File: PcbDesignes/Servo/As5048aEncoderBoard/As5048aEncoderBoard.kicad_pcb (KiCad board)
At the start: 2 copper layers, 8.1 x 11 mm, 8 parts, among them U1 AS5048A-HTSP-500

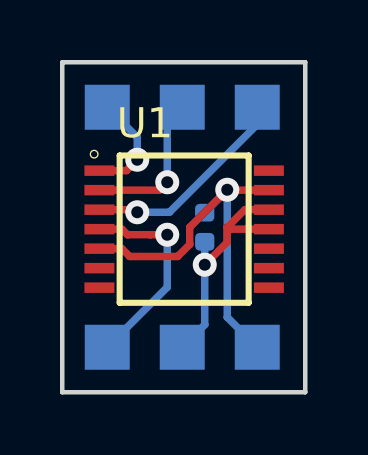
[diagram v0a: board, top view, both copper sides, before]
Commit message: updated schematics and PCB
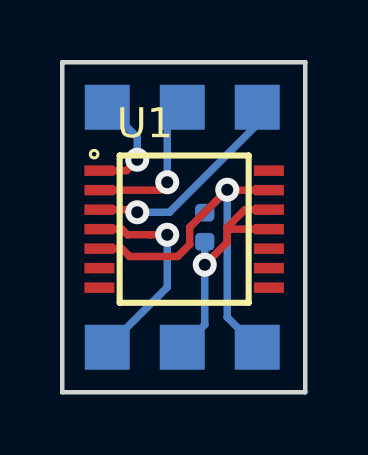
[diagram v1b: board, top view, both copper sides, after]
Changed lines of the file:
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@@
-(kicad_pcb (version 20171130) (host pcbnew 5.0.2+dfsg1-1)
+(kicad_pcb (version 20171130) (host pcbnew 5.1.5+dfsg1-2build2)
   (general
     (thickness 1.6)
@@
     (zone_45_only no)
     (trace_min 0.2)
-    (segment_width 0.2)
-    (edge_width 0.15)
     (via_size 0.8)
     (via_drill 0.4)
@@
     (uvia_min_size 0.2)
     (uvia_min_drill 0.1)
+    (edge_width 0.15)
+    (segment_width 0.2)
     (pcb_text_width 0.3)
     (pcb_text_size 1.5 1.5)
@@
     (fp_line (start 2.15 2.455) (end -2.15 2.455) (layer F.SilkS) (width 0.2032))
     (fp_line (start 2.15 -2.455) (end 2.15 2.455) (layer F.SilkS) (width 0.2032))
-    (fp_circle (center -1.525 -1.825) (end -1.15 -1.825) (layer Eco2.User) (width 0))
+    (fp_circle (center -1.525 -1.825) (end -1.15 -1.825) (layer Eco2.User) (width 0.1))
     (fp_poly (pts (xy -2.22699 -2.10199) (xy -2.22699 -1.79935) (xy -3.20065 -1.79935) (xy -3.20065 -2.10199)) (layer Eco2.User) (width 0))
     (fp_poly (pts (xy -2.22713 -1.45213) (xy -2.22713 -1.14881) (xy -3.20119 -1.14881) (xy -3.20119 -1.45213)) (layer Eco2.User) (width 0))
@@
     (fp_poly (pts (xy 2.22525 -1.15025) (xy 2.22525 -1.44987) (xy 3.20013 -1.44987) (xy 3.20013 -1.15025)) (layer Eco2.User) (width 0))
     (fp_poly (pts (xy 2.22623 -1.80123) (xy 2.22623 -2.09966) (xy 3.20033 -2.09966) (xy 3.20033 -1.80123)) (layer Eco2.User) (width 0))
-    (fp_circle (center -3 -2.5) (end -2.873 -2.5) (layer F.SilkS) (width 0))
+    (fp_circle (center -3 -2.5) (end -2.873 -2.5) (layer F.SilkS) (width 0.1))
     (fp_line (start -3.75 -2.75) (end 3.75 -2.75) (layer Eco1.User) (width 0.127))
     (fp_line (start 3.75 -2.75) (end 3.75 2.75) (layer Eco1.User) (width 0.127))
